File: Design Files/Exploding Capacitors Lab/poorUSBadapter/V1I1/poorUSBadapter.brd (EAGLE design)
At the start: 66 x 13 mm, 12 parts

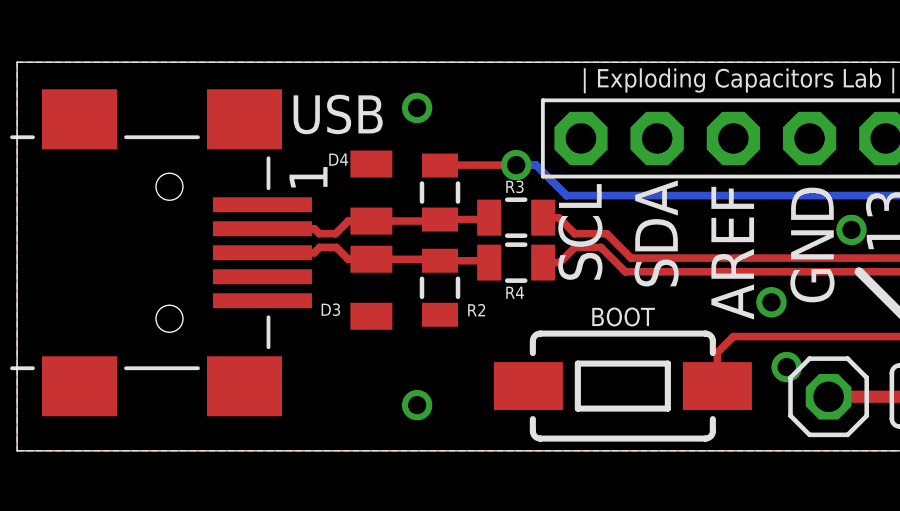
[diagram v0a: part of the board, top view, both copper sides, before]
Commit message: V1I1 is ready!
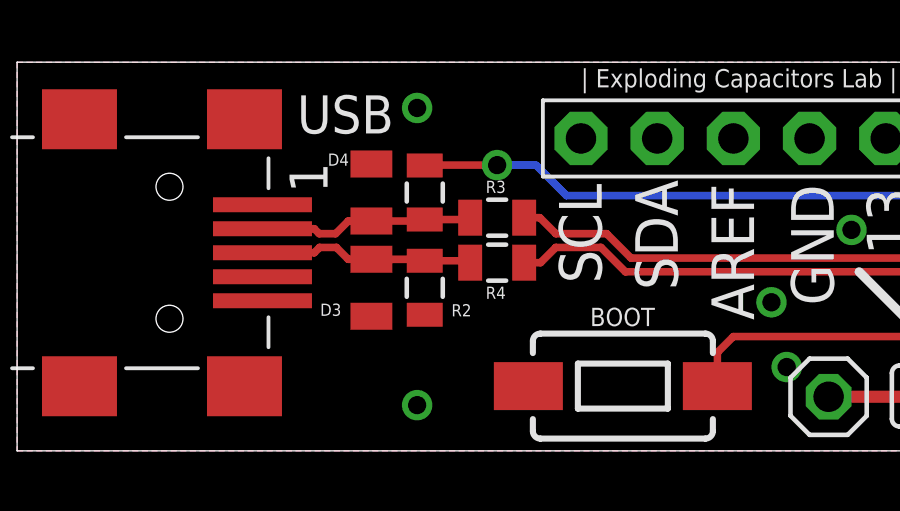
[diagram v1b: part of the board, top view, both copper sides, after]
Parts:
- moved R3 0.64 mm to (16.0, 7.77)
- moved R4 0.64 mm to (16.0, 6.27)
- moved R1 0.51 mm to (13.6, 8.61)
- moved R2 0.51 mm to (13.6, 5.44)
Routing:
- net U_P: track 44.4 -> 45.0 mm
- net U_N: track 43.7 -> 44.3 mm
- net USB_N: track 7.85 -> 7.24 mm
- net USB_P: track 7.84 -> 7.24 mm
- net VCC: track 24.0 -> 24.5 mm
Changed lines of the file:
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@@
 <setting verticaltext="up"/>
 </settings>
-<grid distance="25" unitdist="mil" unit="mil" style="lines" multiple="1" display="yes" altdistance="5" altunitdist="mil" altunit="mil"/>
+<grid distance="5" unitdist="mil" unit="mil" style="lines" multiple="1" display="yes" altdistance="5" altunitdist="mil" altunit="mil"/>
 <layers>
 <layer number="1" name="Top" color="4" fill="1" visible="yes" active="yes"/>
@@
 </autorouter>
 <elements>
-<element name="R1" library="SparkFun-Passives" package="0805" value="1k5" x="14.097" y="8.6106" smashed="yes" rot="R90"/>
-<element name="R2" library="SparkFun-Passives" package="0805" value="1M" x="14.097" y="5.4356" smashed="yes" rot="R90">
-<attribute name="NAME" x="14.986" y="4.4831" size="0.4064" layer="25"/>
-</element>
-<element name="R3" library="SparkFun-Passives" package="0805" value="68R" x="16.637" y="7.7724" smashed="yes">
-<attribute name="NAME" x="16.256" y="8.5979" size="0.4064" layer="25"/>
-</element>
-<element name="R4" library="SparkFun-Passives" package="0805" value="68R" x="16.637" y="6.2738" smashed="yes">
-<attribute name="NAME" x="16.256" y="5.0673" size="0.4064" layer="25"/>
+<element name="R1" library="SparkFun-Passives" package="0805" value="1k5" x="13.589" y="8.6106" smashed="yes" rot="R90"/>
+<element name="R2" library="SparkFun-Passives" package="0805" value="1M" x="13.589" y="5.4356" smashed="yes" rot="R90">
+<attribute name="NAME" x="14.478" y="4.4831" size="0.4064" layer="25"/>
+</element>
+<element name="R3" library="SparkFun-Passives" package="0805" value="68R" x="16.002" y="7.7724" smashed="yes">
+<attribute name="NAME" x="15.621" y="8.5979" size="0.4064" layer="25"/>
+</element>
+<element name="R4" library="SparkFun-Passives" package="0805" value="68R" x="16.002" y="6.2738" smashed="yes">
+<attribute name="NAME" x="15.621" y="5.0673" size="0.4064" layer="25"/>
 </element>
 <element name="USB" library="dp_devices" package="CONN_USB_MINI-B" value="CON-USB-F-MINI-B" x="5.08" y="6.604" smashed="yes" rot="R270">
-<attribute name="NAME" x="9.081" y="10.58" size="1.27" layer="21" font="vector" ratio="10"/>
+<attribute name="NAME" x="9.335" y="10.58" size="1.27" layer="21" font="vector" ratio="10"/>
 </element>
 <element name="BOOT" library="SparkFun-Electromechanical" package="TACTILE-SWITCH-1101NE" value="SWITCH-MOMENTARY-2SMD-1101NE" x="20.193" y="2.159" smashed="yes">
@@
 <contactref element="R4" pad="1"/>
 <contactref element="D3" pad="C"/>
-<wire x1="14.047" y1="6.3856" x2="11.811" y2="6.3856" width="0.254" layer="1"/>
-<wire x1="14.047" y1="6.3856" x2="14.097" y2="6.3356" width="0.254" layer="1"/>
-<wire x1="14.097" y1="6.3356" x2="15.6752" y2="6.3356" width="0.254" layer="1"/>
-<wire x1="15.6752" y1="6.3356" x2="15.737" y2="6.2738" width="0.254" layer="1"/>
+<wire x1="13.589" y1="6.3356" x2="15.0402" y2="6.3356" width="0.254" layer="1"/>
+<wire x1="15.0402" y1="6.3356" x2="15.102" y2="6.2738" width="0.254" layer="1"/>
 <wire x1="8.18" y1="6.604" x2="9.906" y2="6.604" width="0.254" layer="1"/>
 <wire x1="9.906" y1="6.604" x2="10.0838" y2="6.7818" width="0.254" layer="1"/>
-<wire x1="10.6426" y1="6.7818" x2="10.0838" y2="6.7818" width="0.254" layer="1"/>
+<wire x1="10.0838" y1="6.7818" x2="10.6426" y2="6.7818" width="0.254" layer="1"/>
 <wire x1="11.811" y1="6.3856" x2="11.0388" y2="6.3856" width="0.254" layer="1"/>
 <wire x1="11.0388" y1="6.3856" x2="10.6426" y2="6.7818" width="0.254" layer="1"/>
+<wire x1="11.811" y1="6.3856" x2="13.589" y2="6.3856" width="0.254" layer="1"/>
+<wire x1="13.589" y1="6.3856" x2="13.589" y2="6.3356" width="0.254" layer="1"/>
 </signal>
 <signal name="USB_N">
@@
 <contactref element="R3" pad="1"/>
 <contactref element="D4" pad="C"/>
-<wire x1="14.047" y1="7.6606" x2="11.811" y2="7.6606" width="0.254" layer="1"/>
-<wire x1="14.047" y1="7.6606" x2="14.097" y2="7.7106" width="0.254" layer="1"/>
-<wire x1="14.097" y1="7.7106" x2="15.6752" y2="7.7106" width="0.254" layer="1"/>
-<wire x1="15.6752" y1="7.7106" x2="15.737" y2="7.7724" width="0.254" layer="1"/>
+<wire x1="13.589" y1="7.7106" x2="15.0402" y2="7.7106" width="0.254" layer="1"/>
+<wire x1="15.0402" y1="7.7106" x2="15.102" y2="7.7724" width="0.254" layer="1"/>
 <wire x1="8.18" y1="7.404" x2="9.9061" y2="7.404" width="0.254" layer="1"/>
 <wire x1="9.9061" y1="7.404" x2="10.0711" y2="7.239" width="0.254" layer="1"/>
-<wire x1="10.6172" y1="7.239" x2="10.0711" y2="7.239" width="0.254" layer="1"/>
+<wire x1="10.0711" y1="7.239" x2="10.6172" y2="7.239" width="0.254" layer="1"/>
 <wire x1="11.811" y1="7.6606" x2="11.0388" y2="7.6606" width="0.254" layer="1"/>
 <wire x1="11.0388" y1="7.6606" x2="10.6172" y2="7.239" width="0.254" layer="1"/>
+<wire x1="11.811" y1="7.6606" x2="13.589" y2="7.6606" width="0.254" layer="1"/>
+<wire x1="13.589" y1="7.6606" x2="13.589" y2="7.7106" width="0.254" layer="1"/>
 </signal>
 <signal name="GND">
@@
 <wire x1="30.48" y1="8.509" x2="18.3134" y2="8.509" width="0.254" layer="16"/>
 <wire x1="18.3134" y1="8.509" x2="17.2974" y2="9.525" width="0.254" layer="16"/>
-<wire x1="17.2974" y1="9.525" x2="16.637" y2="9.525" width="0.254" layer="16"/>
-<via x="16.637" y="9.525" extent="1-16" drill="0.6096"/>
-<wire x1="16.637" y1="9.525" x2="14.1114" y2="9.525" width="0.254" layer="1"/>
-<wire x1="14.1114" y1="9.525" x2="14.097" y2="9.5106" width="0.254" layer="1"/>
+<wire x1="17.2974" y1="9.525" x2="16.002" y2="9.525" width="0.254" layer="16"/>
+<via x="16.002" y="9.525" extent="1-16" drill="0.6096"/>
+<wire x1="16.002" y1="9.525" x2="14.1114" y2="9.525" width="0.254" layer="1"/>
+<wire x1="14.1114" y1="9.525" x2="13.589" y2="9.5106" width="0.254" layer="1"/>
 </signal>
 <signal name="U_N">
 <contactref element="R3" pad="2"/>
 <contactref element="JP2" pad="5"/>
-<wire x1="17.537" y1="7.7724" x2="18.0594" y2="7.7724" width="0.254" layer="1"/>
-<wire x1="18.0594" y1="7.7724" x2="18.5928" y2="7.239" width="0.254" layer="1"/>
-<wire x1="18.5928" y1="7.239" x2="19.65269375" y2="7.239" width="0.254" layer="1"/>
+<wire x1="16.902" y1="7.7724" x2="17.4244" y2="7.7724" width="0.254" layer="1"/>
+<wire x1="17.4244" y1="7.7724" x2="17.9578" y2="7.239" width="0.254" layer="1"/>
+<wire x1="17.9578" y1="7.239" x2="19.65269375" y2="7.239" width="0.254" layer="1"/>
 <wire x1="19.65269375" y1="7.239" x2="20.46549375" y2="6.4262" width="0.254" layer="1"/>
 <wire x1="52.07690625" y1="6.4262" x2="44.268809375" y2="6.4262" width="0.254" layer="1"/>
@@
 <contactref element="R4" pad="2"/>
 <contactref element="JP2" pad="3"/>
-<wire x1="17.537" y1="6.2738" x2="18.0848" y2="6.2738" width="0.254" layer="1"/>
-<wire x1="18.0848" y1="6.2738" x2="18.5928" y2="6.7818" width="0.254" layer="1"/>
-<wire x1="18.5928" y1="6.7818" x2="19.46330625" y2="6.7818" width="0.254" layer="1"/>
+<wire x1="16.902" y1="6.2738" x2="17.4498" y2="6.2738" width="0.254" layer="1"/>
+<wire x1="17.4498" y1="6.2738" x2="17.9578" y2="6.7818" width="0.254" layer="1"/>
+<wire x1="17.9578" y1="6.7818" x2="19.46330625" y2="6.7818" width="0.254" layer="1"/>
 <wire x1="19.46330625" y1="6.7818" x2="20.27610625" y2="5.969" width="0.254" layer="1"/>
 <wire x1="52.26629375" y1="5.969" x2="20.27610625" y2="5.969" width="0.254" layer="1"/>
